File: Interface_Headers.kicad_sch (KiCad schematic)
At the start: 17 parts, among them J1 BTB_10132798-062100LF, J22 USB_C_Receptacle_USB2.0_16P, J3 SWDB, U7 USBLC6-2SC6

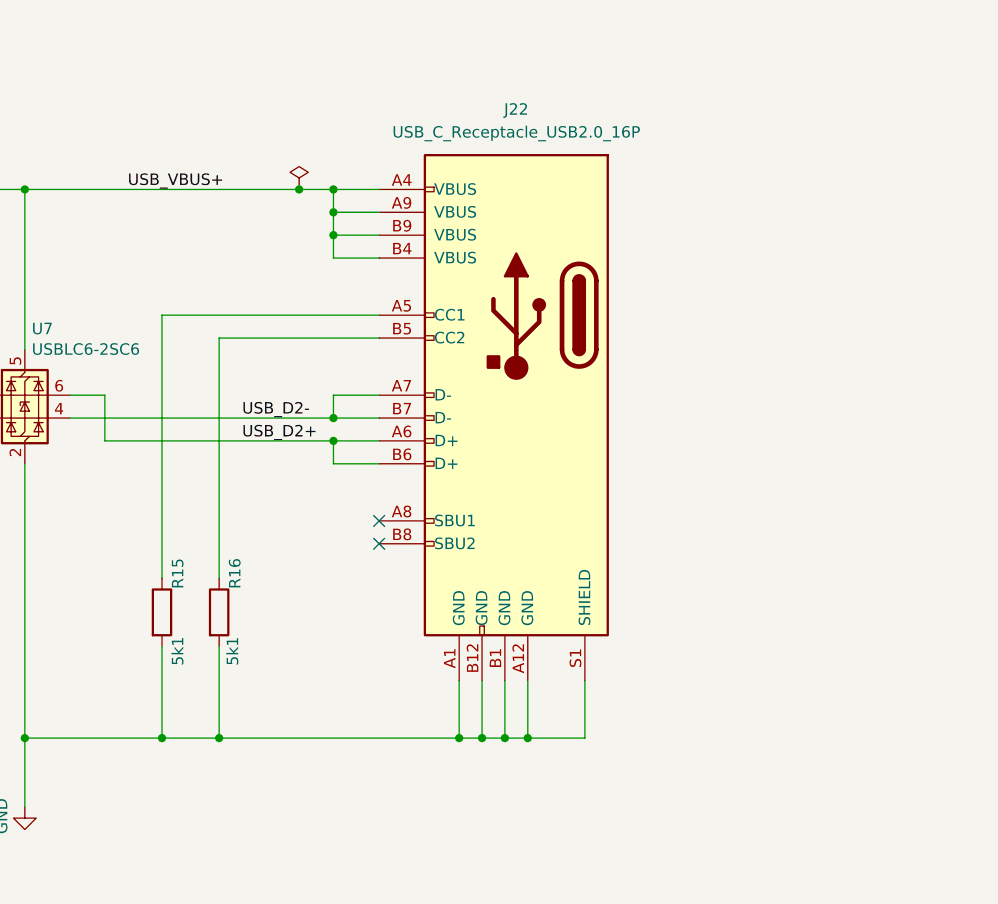
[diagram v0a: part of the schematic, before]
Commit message: Update
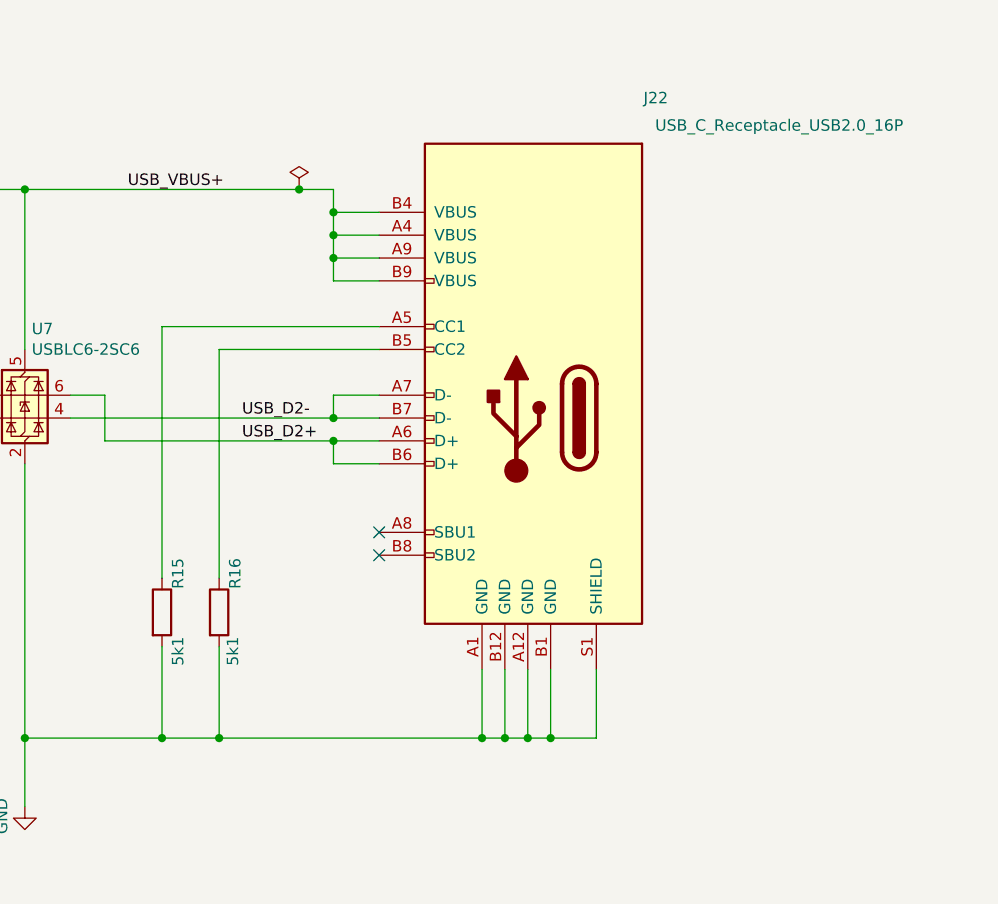
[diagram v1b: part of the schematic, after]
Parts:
- R15, R16: footprint Resistor_SMD:R_0805_2012Metric -> Resistor_SMD:R_0603_1608Metric
